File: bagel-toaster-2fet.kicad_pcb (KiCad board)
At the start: 2 copper layers, 164.2 x 84.2 mm, 118 parts, among them J1 bs, J10 9v, J11 9v, J12 9v, J13 9v, J14 o1b, J15 gnd, J16 gnd, J17 gnd, J18 gnd, J19 i2b, J2 do_snd, J20 o2b, J21 i2, J22 i2s, J23 gnd, J24 o2, J25 9v, J26 o2s, J27 i1, J28 i1s, J29 gnd, J3 out, J30 o1, J31 9v, J32 o1s, J4 in, J5 do_rtn, J6 i1b, J7 bs, J8 gnd, J9 9v, Q1 J113, Q2 J201, SW1 3pdt, SW2 Alpha_3PDT, SW3 Alpha_3PDT, SW4 Alpha_3PDT, U1 TL074, U2 4069

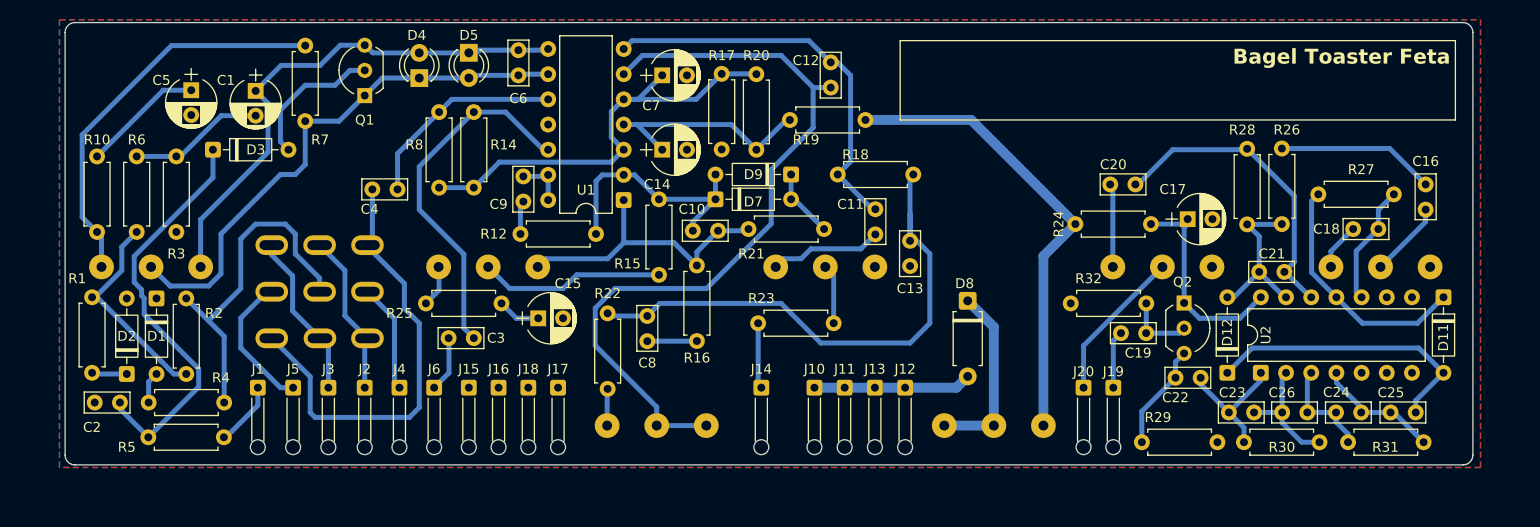
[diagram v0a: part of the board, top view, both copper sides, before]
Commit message: tidier
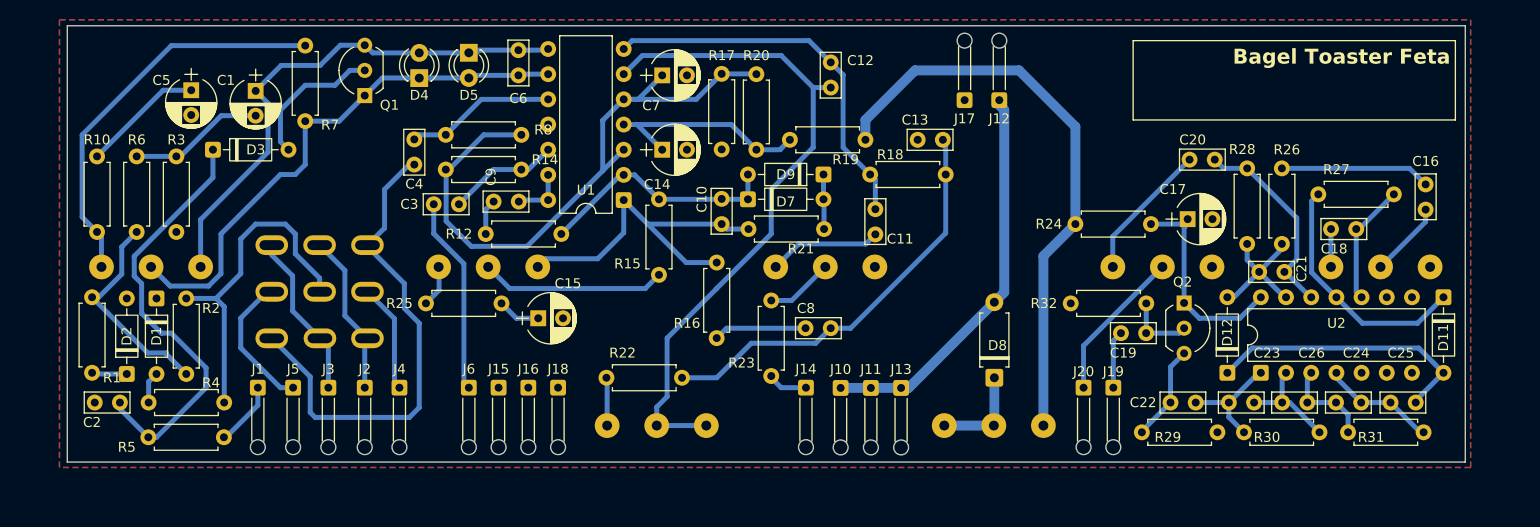
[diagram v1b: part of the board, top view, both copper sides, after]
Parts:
- moved J17 50.2 mm to (156.0, 35.0), turned to 180 degrees
- moved J12 30.5 mm to (159.5, 35.0), turned to 180 degrees
- moved C8 18.5 mm to (142.5, 58.0), turned to 180 degrees
- moved C3 13.6 mm to (102.5, 45.5)
- moved C13 12.8 mm to (151.3, 39.0), turned to 0 degrees
- moved R22 9.92 mm to (127.5, 63.0), turned to 180 degrees
- moved C20 8.38 mm to (181.2, 41.0)
- moved D8 8.21 mm to (159.0, 63.0), turned to 90 degrees
- moved R23 5.49 mm to (136.5, 62.8), turned to 90 degrees
- moved C4 4.91 mm to (100.5, 41.5), turned to 90 degrees
- moved J14 4.50 mm to (140.0, 64.0)
- moved C10 4.33 mm to (131.5, 45.0), turned to -90 degrees
- moved J6 3.50 mm to (106.0, 64.0)
- moved R12 3.50 mm to (115.3, 48.5)
- moved R14 3.36 mm to (103.7, 42.0), turned to 0 degrees
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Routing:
- net Net-(U1D-+): track 36.4 -> 11.3 mm
- net /9v: track 15.9 -> 40.1 mm
- net /vref: track 45.7 -> 65.1 mm
- net Net-(J6-Pin_1): track 5.64 -> 20.0 mm
- net Net-(C13-Pad2): track 54.3 -> 42.2 mm
- net Net-(R19-Pad1): track 47.2 -> 59.1 mm
- net Net-(C20-Pad1): track 31.3 -> 20.4 mm
- net Net-(U1B--): track 79.2 -> 68.6 mm
- net Net-(D8-K): track 18.7 -> 9.84 mm
- net /gainOut: track 29.8 -> 35.8 mm
- net Net-(U1C-+): track 21.1 -> 15.2 mm
- net Net-(C20-Pad2): track 8.43 -> 14.0 mm
- net /b_snd: track 45.1 -> 49.6 mm
- net Net-(C8-Pad2): track 5.01 -> 9.37 mm
- net Net-(J14-Pin_1): track 6.63 -> 4.09 mm
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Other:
- board size 164.2 x 84.2 mm -> 164.2 x 83.9 mm

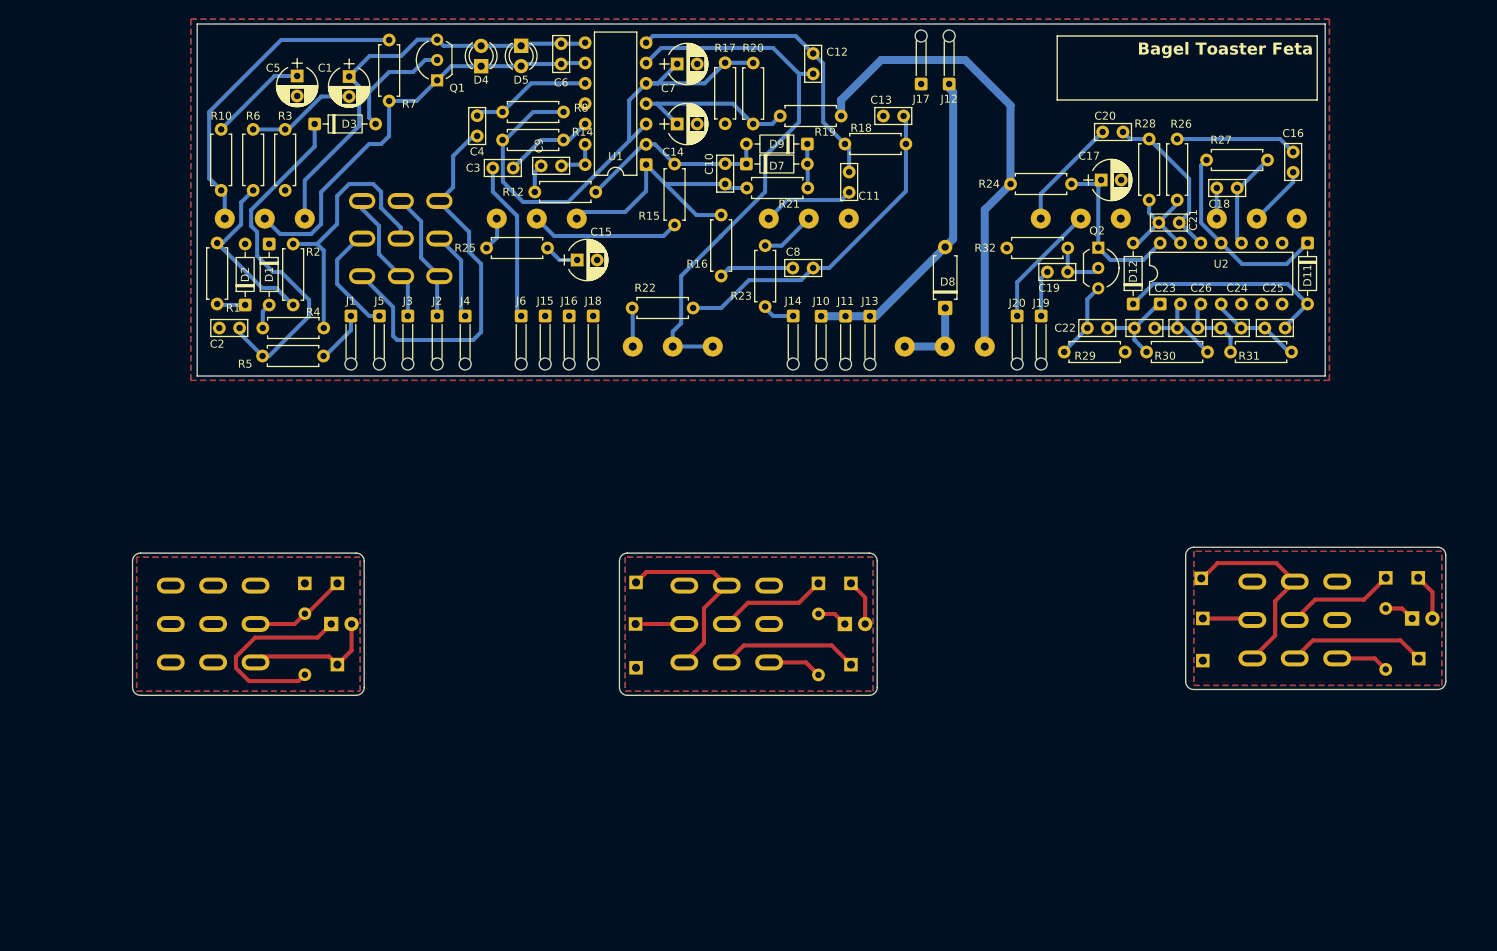
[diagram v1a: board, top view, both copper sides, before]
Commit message: smaller
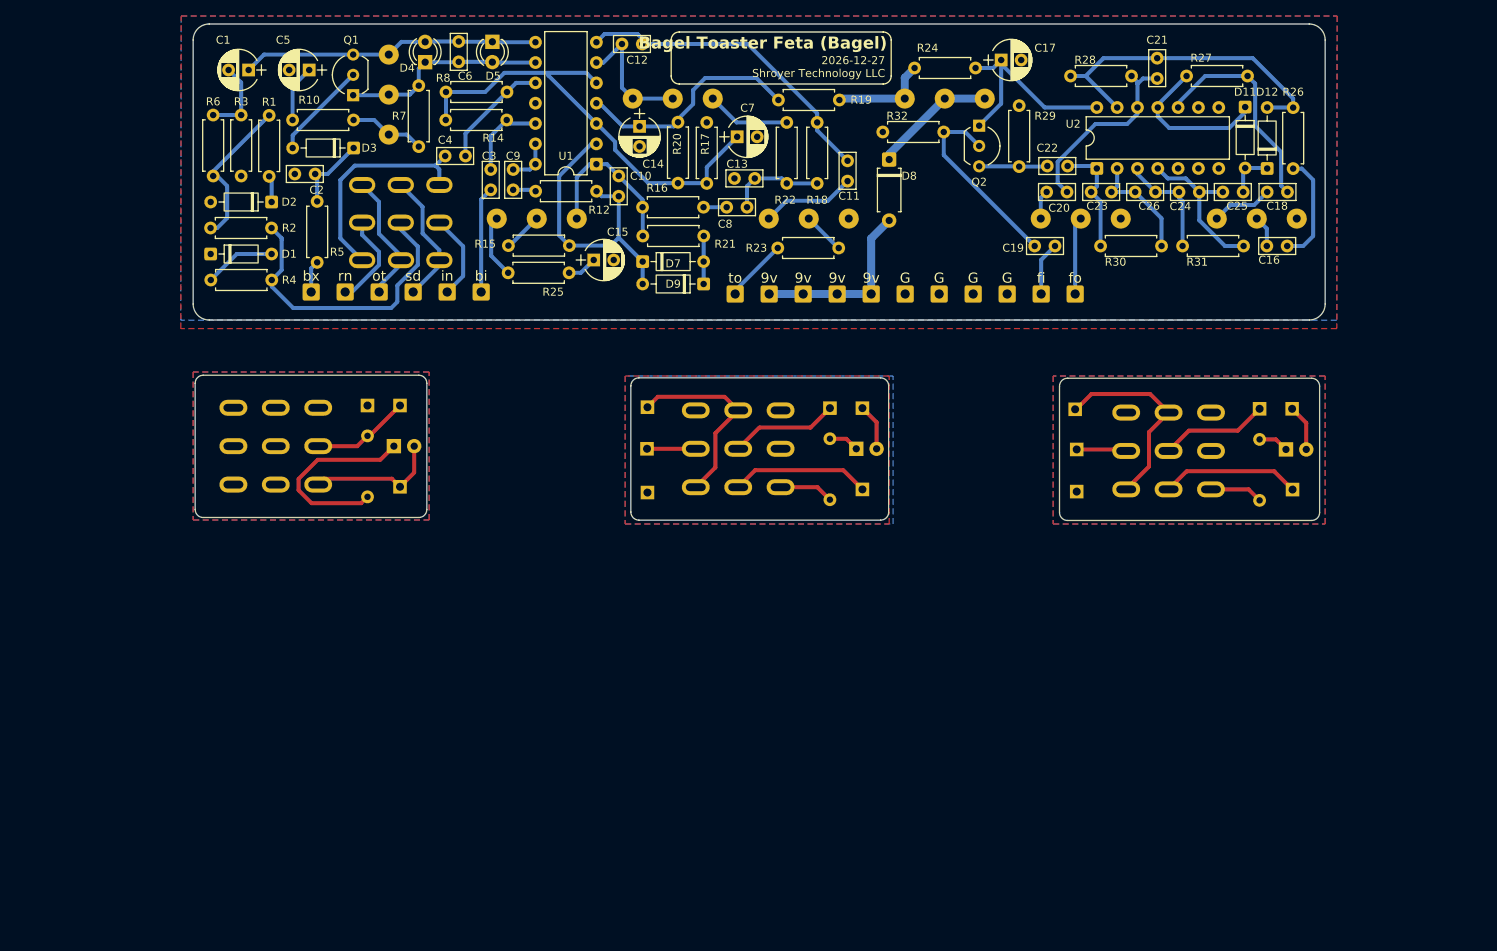
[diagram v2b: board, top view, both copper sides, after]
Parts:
- J1: value bs -> bx; footprint Connector_Wire:SolderWire-0.1sqmm_1x01_D0.4mm_OD1mm_Relief -> Connector_Wire:SolderWire-0.5sqmm_1x01_D0.9mm_OD2.1mm
- J10, J11, J12, J13, J14, J15, J16, J17, J18, J19, J2, J20, J3, J4, J5, J6: footprint Connector_Wire:SolderWire-0.1sqmm_1x01_D0.4mm_OD1mm_Relief -> Connector_Wire:SolderWire-0.5sqmm_1x01_D0.9mm_OD2.1mm
- moved J18 47.6 mm to (162.5, 61.2)
- moved J16 46.3 mm to (158.2, 61.2)
- moved J15 45.1 mm to (154.0, 61.2)
- moved J12 34.6 mm to (137.0, 61.2), turned to 0 degrees
- moved J17 28.4 mm to (166.8, 61.2), turned to 0 degrees
- moved R33 26.4 mm to (198.3, 87.0)
- moved D13 26.4 mm to (201.6, 80.7)
- moved J24 26.4 mm to (198.3, 75.6)
- moved J25 26.4 mm to (202.4, 75.6)
- moved J21 26.4 mm to (175.2, 75.7)
- moved J22 26.4 mm to (175.4, 80.7)
- moved J23 26.4 mm to (175.4, 86.0)
- moved J26 26.4 mm to (202.4, 85.7)
- moved SW3 26.4 mm to (186.9, 80.9)
- moved C12 24.2 mm to (118.6, 30.0), turned to 0 degrees
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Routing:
- net Net-(U1B--): track 68.6 -> 16.5 mm
- net Net-(R19-Pad1): track 59.1 -> 12.6 mm
- net Net-(D3-K): track 43.5 -> 9.68 mm
- net Net-(R10-Pad2): track 40.4 -> 9.53 mm
- net Net-(C13-Pad2): track 42.2 -> 12.1 mm
- net Net-(D4-K): track 54.6 -> 25.8 mm
- net Net-(D12-A): track 15.1 -> 40.8 mm
- net Net-(D11-A): track 28.0 -> 5.88 mm
- net /b_snd: track 49.6 -> 28.1 mm
- net /9v: track 40.1 -> 22.9 mm
- net Net-(Q2-G): track 7.04 -> 24.1 mm
- net Net-(D4-A): track 53.0 -> 37.4 mm
- net /gainOut: track 35.8 -> 20.5 mm
- net Net-(C18-Pad1): track 12.3 -> 27.2 mm
- net Net-(R15-Pad2): track 18.7 -> 4.94 mm
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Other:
- board size 164.2 x 83.9 mm -> 141.5 x 62.1 mm
- board text added: "2026-12-27 Shroyer Technology LLC"
- board text added: "Bagel Toaster Feta (Bagel)"
- board text removed: "Bagel Toaster Feta"

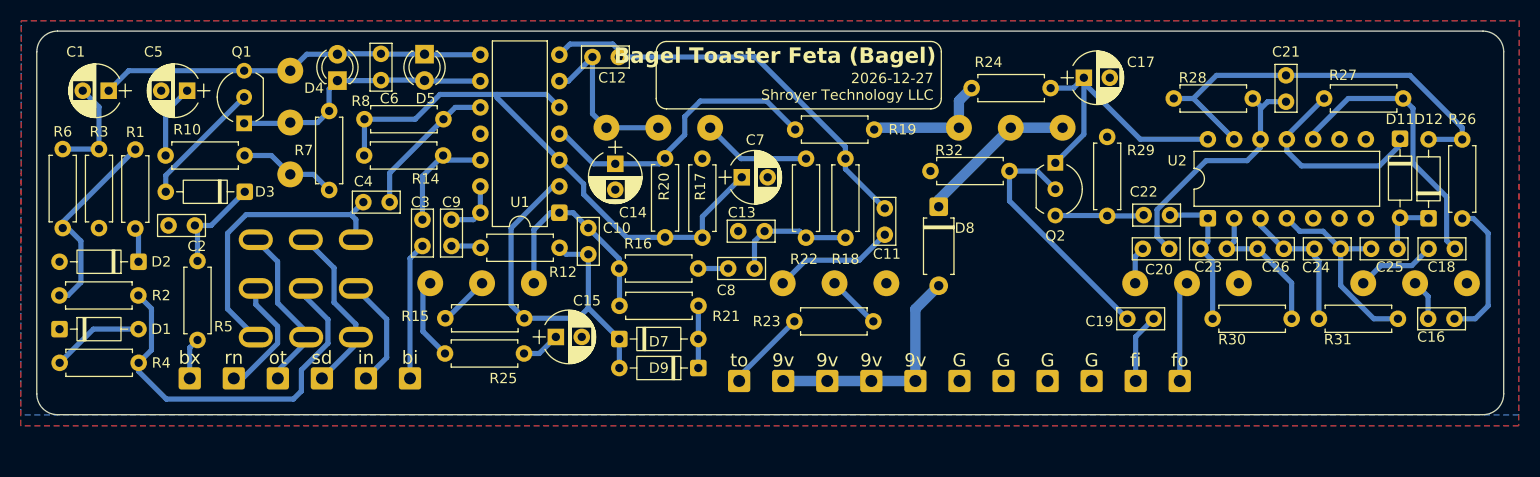
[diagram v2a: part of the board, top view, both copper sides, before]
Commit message: looking pretty good
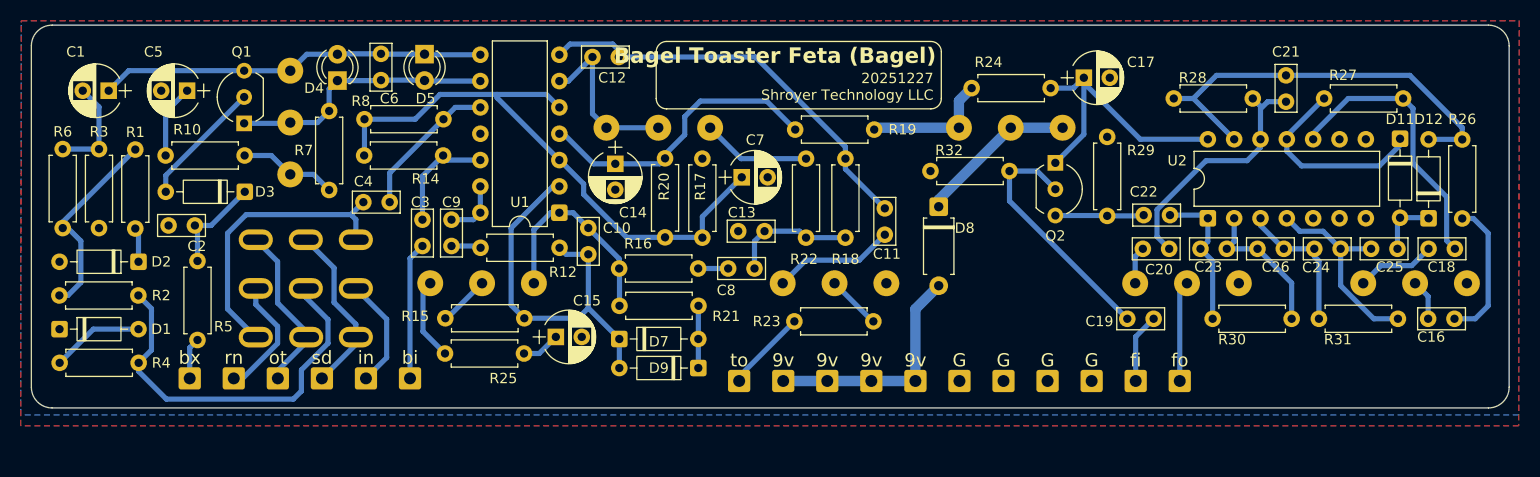
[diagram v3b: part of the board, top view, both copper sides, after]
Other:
- board size 141.5 x 62.1 mm -> 142.6 x 62.6 mm
- board text added: "20251227 Shroyer Technology LLC"
- board text removed: "2026-12-27 Shroyer Technology LLC"
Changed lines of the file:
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@@
+	)
+	(gr_arc
+		(start 205.025 26.925)
+		(mid 206.439214 27.510786)
+		(end 207.025 28.925)
+		(stroke
+			(width 0.05)
+			(type default)
+		)
+		(layer "Edge.Cuts")
 	)
 	(gr_arc
@@
 	)
 	(gr_line
-		(start 67 27.5)
-		(end 204.5 27.5)
-		(stroke
-			(width 0.05)
-			(type default)
-		)
-		(layer "Edge.Cuts")
-	)
-	(gr_line
 		(start 119.716893 72.7335)
 		(end 119.716893 88.5135)
-		(stroke
-			(width 0.05)
-			(type default)
-		)
-		(layer "Edge.Cuts")
-	)
-	(gr_arc
-		(start 65 29.5)
-		(mid 65.585786 28.085786)
-		(end 67 27.5)
 		(stroke
 			(width 0.05)
@@
 		(layer "Edge.Cuts")
 	)
-	(gr_line
-		(start 206.5 29.5)
-		(end 206.5 62.5)
-		(stroke
-			(width 0.05)
-			(type default)
-		)
-		(layer "Edge.Cuts")
-	)
-	(gr_line
-		(start 65 62.5)
-		(end 65 29.5)
-		(stroke
-			(width 0.05)
-			(type default)
-		)
-		(layer "Edge.Cuts")
-	)
-	(gr_arc
-		(start 206.5 62.5)
-		(mid 205.914214 63.914214)
-		(end 204.5 64.5)
+	(gr_arc
+		(start 66.475 63.85)
+		(mid 65.060786 63.264214)
+		(end 64.475 61.85)
+		(stroke
+			(width 0.05)
+			(type default)
+		)
+		(layer "Edge.Cuts")
+	)
+	(gr_line
+		(start 64.475 61.85)
+		(end 64.475 28.925)
 		(stroke
 			(width 0.05)
@@
 	)
 	(gr_arc
-		(start 67 64.5)
-		(mid 65.585786 63.914214)
-		(end 65 62.5)
-		(stroke
-			(width 0.05)
-			(type default)
-		)
-		(layer "Edge.Cuts")
-	)
-	(gr_arc
 		(start 65.252 72.406)
 		(mid 65.544893 71.698893)
@@
 	)
 	(gr_line
-		(start 204.5 64.5)
-		(end 67 64.5)
+		(start 205.025 63.85)
+		(end 66.475 63.85)
+		(stroke
+			(width 0.05)
+			(type default)
+		)
+		(layer "Edge.Cuts")
+	)
+	(gr_line
+		(start 66.475 26.925)
+		(end 205.025 26.925)
 		(stroke
 			(width 0.05)
@@
 		(start 120.716893 89.5135)
 		(end 150.936 89.5135)
+		(stroke
+			(width 0.05)
+			(type default)
+		)
+		(layer "Edge.Cuts")
+	)
+	(gr_line
+		(start 207.025 28.925)
+		(end 207.025 61.85)
 		(stroke
 			(width 0.05)
@@
 	)
 	(gr_arc
-		(start 204.5 27.5)
-		(mid 205.914214 28.085786)
-		(end 206.5 29.5)
+		(start 64.475 28.925)
+		(mid 65.060786 27.510786)
+		(end 66.475 26.925)
 		(stroke
 			(width 0.05)
@@
 		(layer "Edge.Cuts")
 	)
-	(gr_text "2026-12-27\nShroyer Technology LLC\n"
+	(gr_arc
+		(start 207.025 61.85)
+		(mid 206.439214 63.264214)
+		(end 205.025 63.85)
+		(stroke
+			(width 0.05)
+			(type default)
+		)
+		(layer "Edge.Cuts")
+	)
+	(gr_text "20251227\nShroyer Technology LLC\n"
 		(at 151.5 34.25 0)
 		(layer "F.SilkS")
@@
 		(layer "Cmts.User")
 		(pts
-			(xy 65.5 27.5) (xy 206.5 27.5)
-		)
-		(height -10.6)
+			(xy 173.296 72.778) (xy 205.808 72.778)
+		)
+		(height -3.728)
 		(orientation 0)
 		(format
@@
 			(keep_text_aligned yes)
 		)
-		(gr_text "141"
-			(at 136 15.75 0)
+		(gr_text "32.512"
+			(at 189.552 67.9 0)
 			(layer "Cmts.User")
 			(effects
@@
 		(layer "Cmts.User")
 		(pts
-			(xy 206.5 27.5) (xy 206.5 71.5)
-		)
-		(height 11.86)
+			(xy 205.025 63.85) (xy 205.025 26.925)
+		)
+		(height 7.225)
 		(orientation 1)
 		(format
@@
 			(keep_text_aligned yes)
 		)
-		(gr_text "44"
-			(at 217.21 49.5 90)
+		(gr_text "36.925"
+			(at 211.1 45.3875 90)
 			(layer "Cmts.User")
 			(effects
+				(font
+					(size 1 1)
+					(thickness 0.15)
+				)
+			)
+		)
+	)
+	(dimension
+		(type orthogonal)
+		(layer "Cmts.User")
+		(pts
+			(xy 207.025 28.925) (xy 64.475 28.925)
+		)
+		(height -9.55)
+		(orientation 0)
+		(format
+			(prefix "")
+			(suffix "")
+			(units 3)
+			(units_format 0)
+			(precision 4)
+			(suppress_zeroes yes)
+		)
+		(style
+			(thickness 0.1)
+			(arrow_length 1.27)
+			(text_position_mode 0)
+			(arrow_direction outward)
+			(extension_height 0.58642)
+			(extension_offset 0.5)
+			(keep_text_aligned yes)
+		)
+		(gr_text "142.55"
+			(at 135.75 18.225 0)
+			(layer "Cmts.User")
+			(effects
